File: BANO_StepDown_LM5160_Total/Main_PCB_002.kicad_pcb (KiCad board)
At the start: 2 copper layers, 27 parts, among them U1 LM5160ADNTR, U2 TLV9061IDCKR

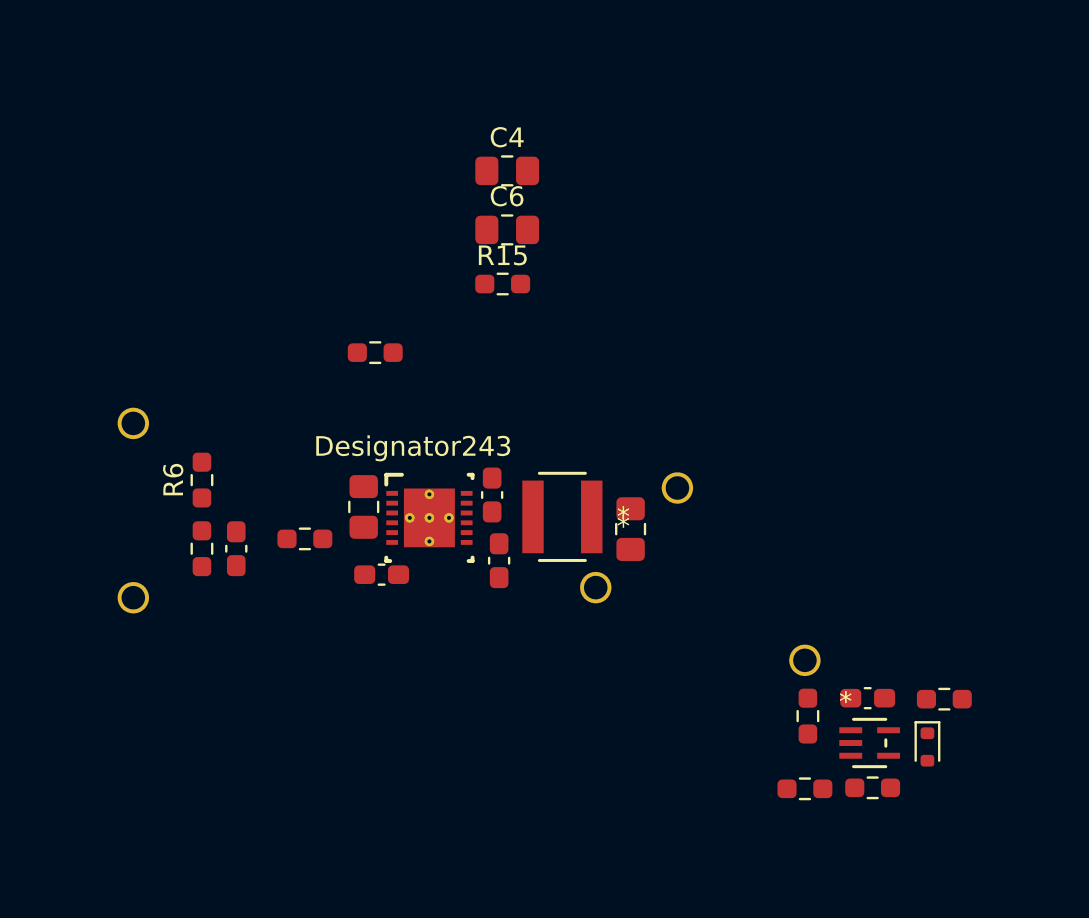
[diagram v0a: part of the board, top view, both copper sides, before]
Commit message: BANO Step-Dn 004
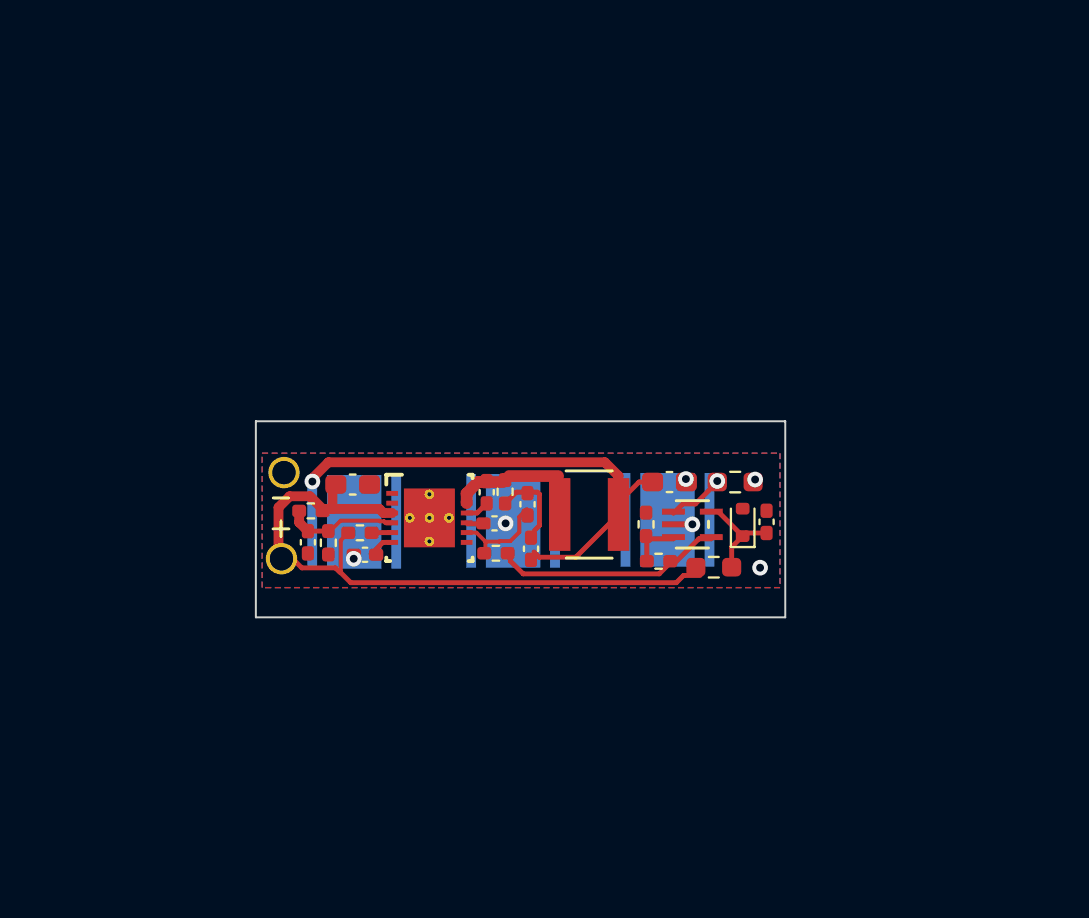
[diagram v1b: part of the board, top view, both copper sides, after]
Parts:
- removed D1, D2: WireHole_1p5, Wire_holes:WireHole_1p2
- added D6: LED_Cree_XHP50_6V, LED_SMD:LED_Cree-XHP50_6V, B.Cu at (120.0, 122.6)
- added D8: LED_Cree_XHP50_6V, LED_SMD:LED_Cree-XHP50_6V, B.Cu at (136.0, 122.5)
- C1, C2, C26, C27, C3: footprint Capacitor_SMD:C_0603_1608Metric_Pad1.08x0.95mm_HandSolder -> Capacitor_SMD:C_0402_1005Metric_Pad0.74x0.62mm_HandSolder
- C28, C5: footprint Capacitor_SMD:C_0805_2012Metric_Pad1.18x1.45mm_HandSolder -> Capacitor_SMD:C_0603_1608Metric_Pad1.08x0.95mm_HandSolder
- C4, C6: footprint Capacitor_SMD:C_0805_2012Metric_Pad1.18x1.45mm_HandSolder -> Capacitor_SMD:C_0402_1005Metric_Pad0.74x0.62mm_HandSolder
- D7: value WireHole_1p5 -> LED_Cree_XHP50_6V; footprint Wire_holes:WireHole_1p2 -> LED_SMD:LED_Cree-XHP50_6V; moved to B.Cu
- R1, R15, R3, R4, R6, R7, R9: footprint Resistor_SMD:R_0603_1608Metric_Pad0.98x0.95mm_HandSolder -> Resistor_SMD:R_0402_1005Metric_Pad0.72x0.64mm_HandSolder
- moved C4 19.3 mm to (129.0, 124.0), turned to 90 degrees
- moved R3 15.9 mm to (135.5, 124.6)
- moved R4 15.7 mm to (134.9, 122.8), turned to -90 degrees
- moved D23 14.8 mm to (139.8, 122.7), turned to 90 degrees
- moved U2 14.4 mm to (137.3, 122.8)
- moved C6 14.0 mm to (128.9, 121.7), turned to -90 degrees
- moved R15 13.7 mm to (127.2, 124.2), turned to 180 degrees
- moved R5 13.6 mm to (138.4, 124.9), turned to 180 degrees
- moved R2 12.5 mm to (139.4, 120.6), turned to 0 degrees
- moved C1 10.4 mm to (141.0, 122.6), turned to 90 degrees
- moved D27 10.2 mm to (116.3, 124.5)
- moved D28 9.99 mm to (116.4, 120.1)
- moved R1 9.71 mm to (127.7, 121.1), turned to 90 degrees
- moved R7 6.45 mm to (118.7, 123.7)
- moved R6 5.77 mm to (117.8, 122.1), turned to 0 degrees
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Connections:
- C2 pad 1: Net-(D7-Conn) -> Net-(U1-VCC)
- D7 pad 1: Net-(D7-Conn) -> Net-(D7-K)
- U1 pad 9: Net-(D7-Conn) -> Net-(U1-VCC)
- U1 pad V: (no net) -> GND2
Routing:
- net Net-(D27-Conn): track 0.00 -> 34.4 mm
- net Net-(D6-A): track 0.00 -> 26.6 mm, vias 0 -> 1
- net Net-(U2-OUT): track 0.00 -> 11.6 mm
- net Net-(C27-Pad2): track 0.00 -> 8.81 mm
- net Net-(U1-EN_UVLO): track 0.00 -> 6.08 mm
- net Net-(D23-K): track 0.00 -> 5.44 mm
- net Net-(U1-FB): track 0.00 -> 5.06 mm
- net Net-(C4-Pad2): track 0.00 -> 3.99 mm
- net Net-(D8-K): track 0.00 -> 3.08 mm, vias 0 -> 1
- net Net-(U2-IN-): track 0.00 -> 2.49 mm
- net Net-(U1-SS): track 0.00 -> 1.32 mm
- net Net-(U1-BST): track 0.00 -> 1.22 mm
- net Net-(U1-RON): track 0.00 -> 1.10 mm
- net Net-(U1-VCC): track 0.00 -> 1.05 mm
- net GND2: vias 0 -> 6
- added copper zone on B.Cu, net GND2
- added copper zone on F.Cu, net GND2
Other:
- board outline added: 27 x 10 mm
